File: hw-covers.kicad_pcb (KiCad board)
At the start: 2 copper layers, 122 x 70 mm, 117 parts, among them J1 Screw_Terminal_01x04, J10 Screw_Terminal_01x03, J11 Screw_Terminal_01x03, J2 Screw_Terminal_01x04, J3 Conn_01x04_Pin, J4 Conn_01x04_Pin, J5 Screw_Terminal_01x03, J6 Conn_01x02_Pin, J7 Screw_Terminal_01x04, J8 Screw_Terminal_01x03, J9 Screw_Terminal_01x03, K1 JRC-21F(4100), K10 JRC-21F(4100), K2 JRC-21F(4100), K3 JRC-21F(4100), K4 JRC-21F(4100), K5 JRC-21F(4100), K6 JRC-21F(4100), K7 JRC-21F(4100), K8 JRC-21F(4100), K9 JRC-21F(4100), Q1 PMBT3904235, Q10 PMBT3904235, Q11 PMBT3904235, Q2 PMBT3904235, Q3 PMBT3904235, Q4 PMBT3904235, Q5 PMBT3904235, Q6 PMBT3904235, Q7 PMBT3904235, Q8 PMBT3904235, Q9 PMBT3904235, SW1 SW_Push, U1 ESP32-S3-WROOM-1, U2 NCP1117-3.3_SOT223, U3 HLK-2M05

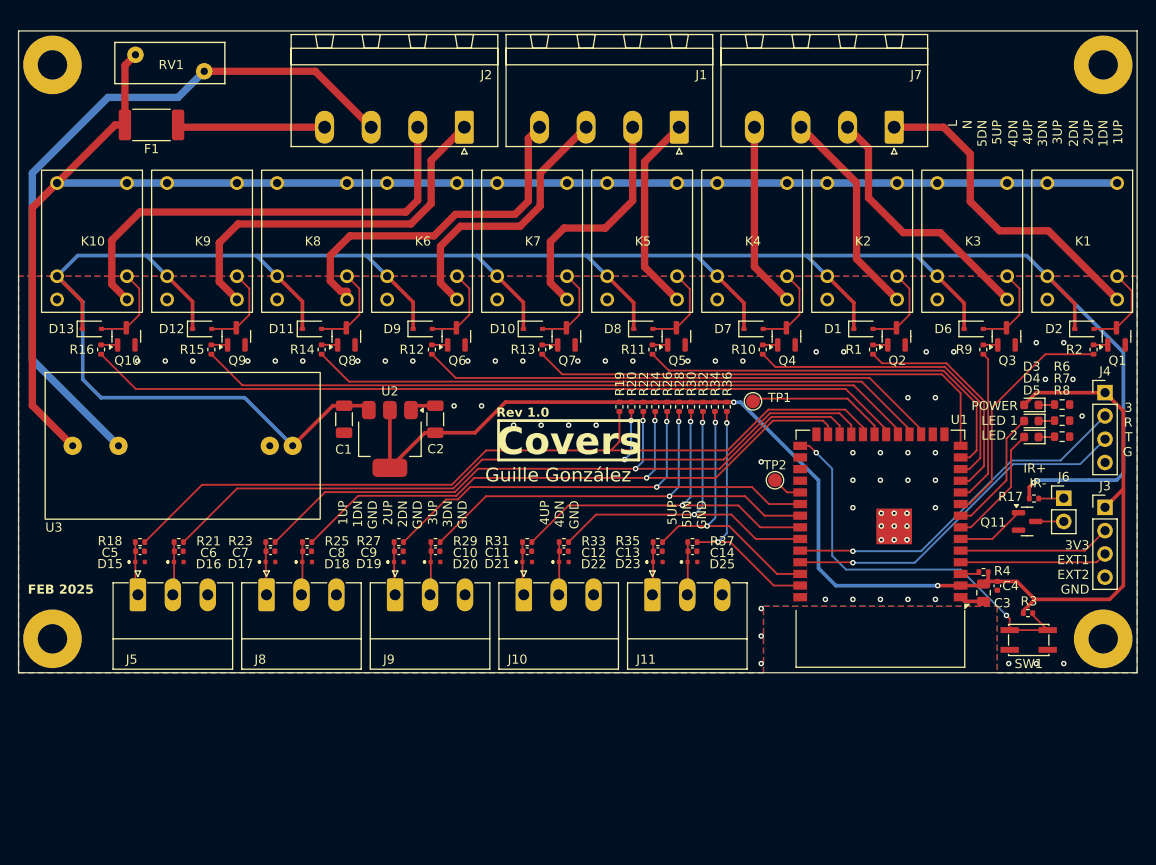
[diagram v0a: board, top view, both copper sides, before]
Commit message: Release 1.1
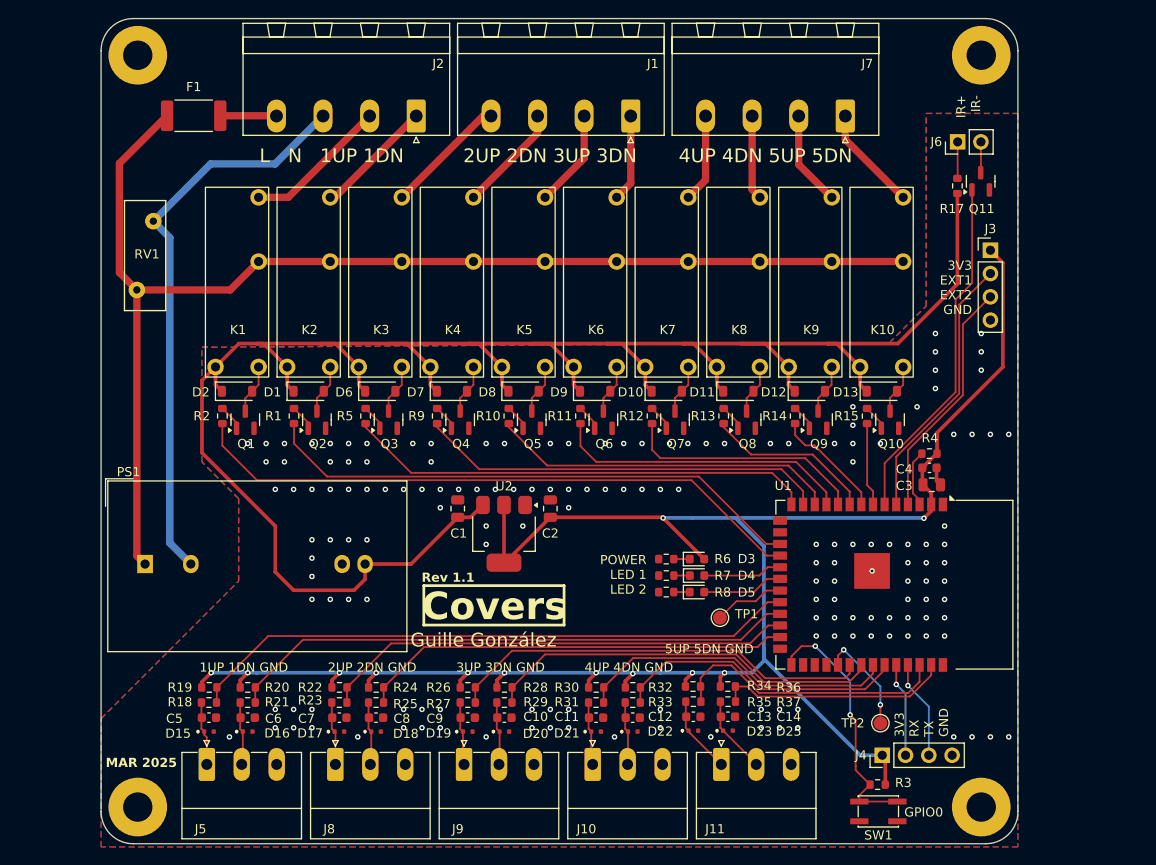
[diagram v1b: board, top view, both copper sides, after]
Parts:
- removed R16: 1k, Resistor_SMD:R_0402_1005Metric
- removed U3: HLK-2M05, guille-lib:HLK-2M05
- added PS1: HLK-2M05, Converter_ACDC:Converter_ACDC_Hi-Link_HLK-2Mxx, F.Cu at (108.8, 110.1)
- added R5: 1k, Resistor_SMD:R_0603_1608Metric, F.Cu at (132.9, 94.0)
- C1, C2: footprint Capacitor_SMD:C_1206_3216Metric -> Capacitor_SMD:C_0805_2012Metric
- C10, C11, C12, C13, C14, C4, C5, C6, C7, C8, C9: footprint Capacitor_SMD:C_0402_1005Metric -> Capacitor_SMD:C_0603_1608Metric
- D1, D10, D11, D12, D13, D2, D6, D7, D8, D9: footprint Diode_SMD:D_SOD-323 -> Diode_SMD:D_SOD-123
- K1, K10, K2, K3, K4, K5, K6, K7, K8, K9: value JRC-21F(4100) -> HF46F; footprint guille-lib:JRC-21F(4100) -> guille-lib:HF46F
- R1, R10, R11, R12, R13, R14, R15, R17, R18, R19, R2, R20, R21, R22, R23, R24, R25, R26, R27, R28, R29, R3, R30, R31, R32, R33, R34, R35, R36, R37, R4, R9: footprint Resistor_SMD:R_0402_1005Metric -> Resistor_SMD:R_0603_1608Metric
- moved Q1 95.5 mm to (119.7, 94.4)
- moved R2 95.3 mm to (117.2, 94.0)
- moved D2 92.7 mm to (118.8, 91.3)
- moved K1 90.9 mm to (121.2, 88.7), turned to 90 degrees
- moved K10 89.5 mm to (191.5, 88.7), turned to 90 degrees
- moved D13 86.4 mm to (189.2, 91.3)
- moved Q10 83.8 mm to (190.1, 94.4)
- moved R15 71.9 mm to (187.6, 94.0)
- moved K9 70.1 mm to (183.7, 88.7), turned to 90 degrees
- moved Q3 68.0 mm to (135.4, 94.4)
- moved D12 66.6 mm to (181.3, 91.3)
- moved D6 65.1 mm to (134.5, 91.3)
- moved Q9 64.1 mm to (182.2, 94.4)
- moved Q2 63.9 mm to (127.5, 94.4)
- moved K3 63.7 mm to (136.8, 88.7), turned to 90 degrees
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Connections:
- J1 pad 1: /OUT3_UP -> /OUT3_DOWN
- J1 pad 2: /OUT3_DOWN -> /OUT3_UP
- J1 pad 3: /OUT4_UP -> /OUT2_DOWN
- J1 pad 4: /OUT4_DOWN -> /OUT2_UP
- J2 pad 1: /OUT5_UP -> /OUT1_DOWN
- J2 pad 2: /OUT5_DOWN -> /OUT1_UP
- J7 pad 1: /OUT1_UP -> /OUT5_DOWN
- J7 pad 2: /OUT1_DOWN -> /OUT5_UP
- J7 pad 3: /OUT2_UP -> /OUT4_DOWN
- J7 pad 4: /OUT2_DOWN -> /OUT4_UP
- K1 pad 1: /LF -> /OUT1_UP
- K1 pad 2: +5V -> /LF
- K1 pad 3: unconnected-(K1-NC-Pad3) -> Net-(D2-A)
- K1 pad 4: /OUT1_UP -> +5V
- K10 pad 1: /LF -> /OUT5_DOWN
- K10 pad 2: +5V -> /LF
- K10 pad 3: unconnected-(K10-NC-Pad3) -> Net-(D13-A)
- K10 pad 4: /OUT5_DOWN -> +5V
- K2 pad 1: /LF -> /OUT1_DOWN
- K2 pad 2: +5V -> /LF
- K2 pad 3: unconnected-(K2-NC-Pad3) -> Net-(D1-A)
- K2 pad 4: /OUT2_UP -> +5V
- K3 pad 1: /LF -> /OUT2_UP
- K3 pad 2: +5V -> /LF
- K3 pad 3: unconnected-(K3-NC-Pad3) -> Net-(D6-A)
- K3 pad 4: /OUT1_DOWN -> +5V
- K4 pad 1: /LF -> /OUT2_DOWN
- K4 pad 2: +5V -> /LF
- K4 pad 3: unconnected-(K4-NC-Pad3) -> Net-(D7-A)
- K4 pad 4: /OUT2_DOWN -> +5V
- K5 pad 1: /LF -> /OUT3_UP
- K5 pad 2: +5V -> /LF
- K5 pad 3: unconnected-(K5-NC-Pad3) -> Net-(D8-A)
- K5 pad 4: /OUT3_UP -> +5V
- K6 pad 1: /LF -> /OUT3_DOWN
- K6 pad 2: +5V -> /LF
- K6 pad 3: unconnected-(K6-NC-Pad3) -> Net-(D9-A)
- K6 pad 4: /OUT4_UP -> +5V
- K7 pad 1: /LF -> /OUT4_UP
- K7 pad 2: +5V -> /LF
- K7 pad 3: unconnected-(K7-NC-Pad3) -> Net-(D10-A)
- K7 pad 4: /OUT3_DOWN -> +5V
- K8 pad 1: /LF -> /OUT4_DOWN
- K8 pad 2: +5V -> /LF
- K8 pad 3: unconnected-(K8-NC-Pad3) -> Net-(D11-A)
- K8 pad 4: /OUT4_DOWN -> +5V
- K9 pad 1: /LF -> /OUT5_UP
- K9 pad 2: +5V -> /LF
- K9 pad 3: unconnected-(K9-NC-Pad3) -> Net-(D12-A)
- K9 pad 4: /OUT5_UP -> +5V
- R1 pad 1: /2OUT1 -> /1OUT2
- R10 pad 1: /2OUT2 -> /3OUT1
- R10 pad 2: Net-(Q4-Pad1) -> Net-(Q5-Pad1)
- R11 pad 1: /3OUT1 -> /3OUT2
- R11 pad 2: Net-(Q5-Pad1) -> Net-(Q6-Pad1)
- R12 pad 2: Net-(Q6-Pad1) -> Net-(Q7-Pad1)
- R13 pad 1: /3OUT2 -> /4OUT2
- R13 pad 2: Net-(Q7-Pad1) -> Net-(Q8-Pad1)
- R14 pad 1: /4OUT2 -> /5OUT1
- R14 pad 2: Net-(Q8-Pad1) -> Net-(Q9-Pad1)
- R15 pad 1: /5OUT1 -> /5OUT2
- R15 pad 2: Net-(Q9-Pad1) -> Net-(Q10-Pad1)
- R9 pad 1: /1OUT2 -> /2OUT2
- R9 pad 2: Net-(Q3-Pad1) -> Net-(Q4-Pad1)
- U1 pad 10: /1OUT2 -> /4OUT1
- U1 pad 11: /2OUT1 -> /3OUT2
- U1 pad 12: /2OUT2 -> /3OUT1
- U1 pad 13: /3OUT1 -> /2OUT2
- U1 pad 14: /3OUT2 -> /2OUT1
- U1 pad 17: /4OUT1 -> /1OUT2
- U1 pad 18: /4OUT2 -> /1OUT1
- U1 pad 19: /5OUT1 -> /LED1
- U1 pad 20: /5OUT2 -> /LED2
- U1 pad 7: /LED2 -> /5OUT2
- U1 pad 8: /LED1 -> /5OUT1
- U1 pad 9: /1OUT1 -> /4OUT2
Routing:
- net /5OUT2: track 89.6 -> 9.09 mm
- net +3V3: track 142.4 -> 213.2 mm, vias 2 -> 12
- net /5OUT1: track 78.8 -> 12.4 mm
- net +5V: track 290.1 -> 224.6 mm, vias 1 -> 0
- net /4OUT2: track 68.1 -> 18.5 mm
- net /1OUT2: track 17.1 -> 59.7 mm
- net /1OUT1: track 26.0 -> 68.2 mm
- net /OUT5_DOWN: track 50.3 -> 11.5 mm
- net /OUT5_UP: track 41.7 -> 10.4 mm
- net /4OUT1: track 57.3 -> 26.5 mm
- net /IR: track 7.50 -> 38.3 mm
- net /OUT4_DOWN: track 38.6 -> 9.22 mm
- net /ESP_RX: track 39.4 -> 10.3 mm
- net /LF: track 165.4 -> 137.1 mm
- net /ESP_TX: track 38.9 -> 10.8 mm
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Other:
- board size 122 x 70 mm -> 100 x 90 mm
- board text added: "1DN 1UP N L"
- board text added: "2UP 2DN 3UP 3DN"
- board text added: "3DN 3UP 2DN 2UP"
- board text added: "4UP 4DN 5UP 5DN"
- board text added: "5DN 5UP 4DN 4UP"
- board text added: "GPIO0"
- board text added: "IR- IR+"
- board text added: "L N 1UP 1DN"
- board text added: "MAR 2025"
- board text added: "Rev 1.1"
- board text removed: "1UP 1DN 2UP 2DN"
- board text removed: "2DN 2UP 1DN 1UP"
- board text removed: "3 R T G"
- board text removed: "3UP 3DN 4UP 4DN"
- board text removed: "4DN 4UP 3DN 3UP"
- board text removed: "5UP 5DN N L"
- board text removed: "FEB 2025"
- board text removed: "L N 5DN 5UP"
- board text removed: "Rev 1.0"
